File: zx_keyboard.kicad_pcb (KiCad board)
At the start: 2 copper layers, 194.3 x 127 mm, 3 parts, among them SW1 SW_PUSH, SW2 SW_PUSH, U1 4066

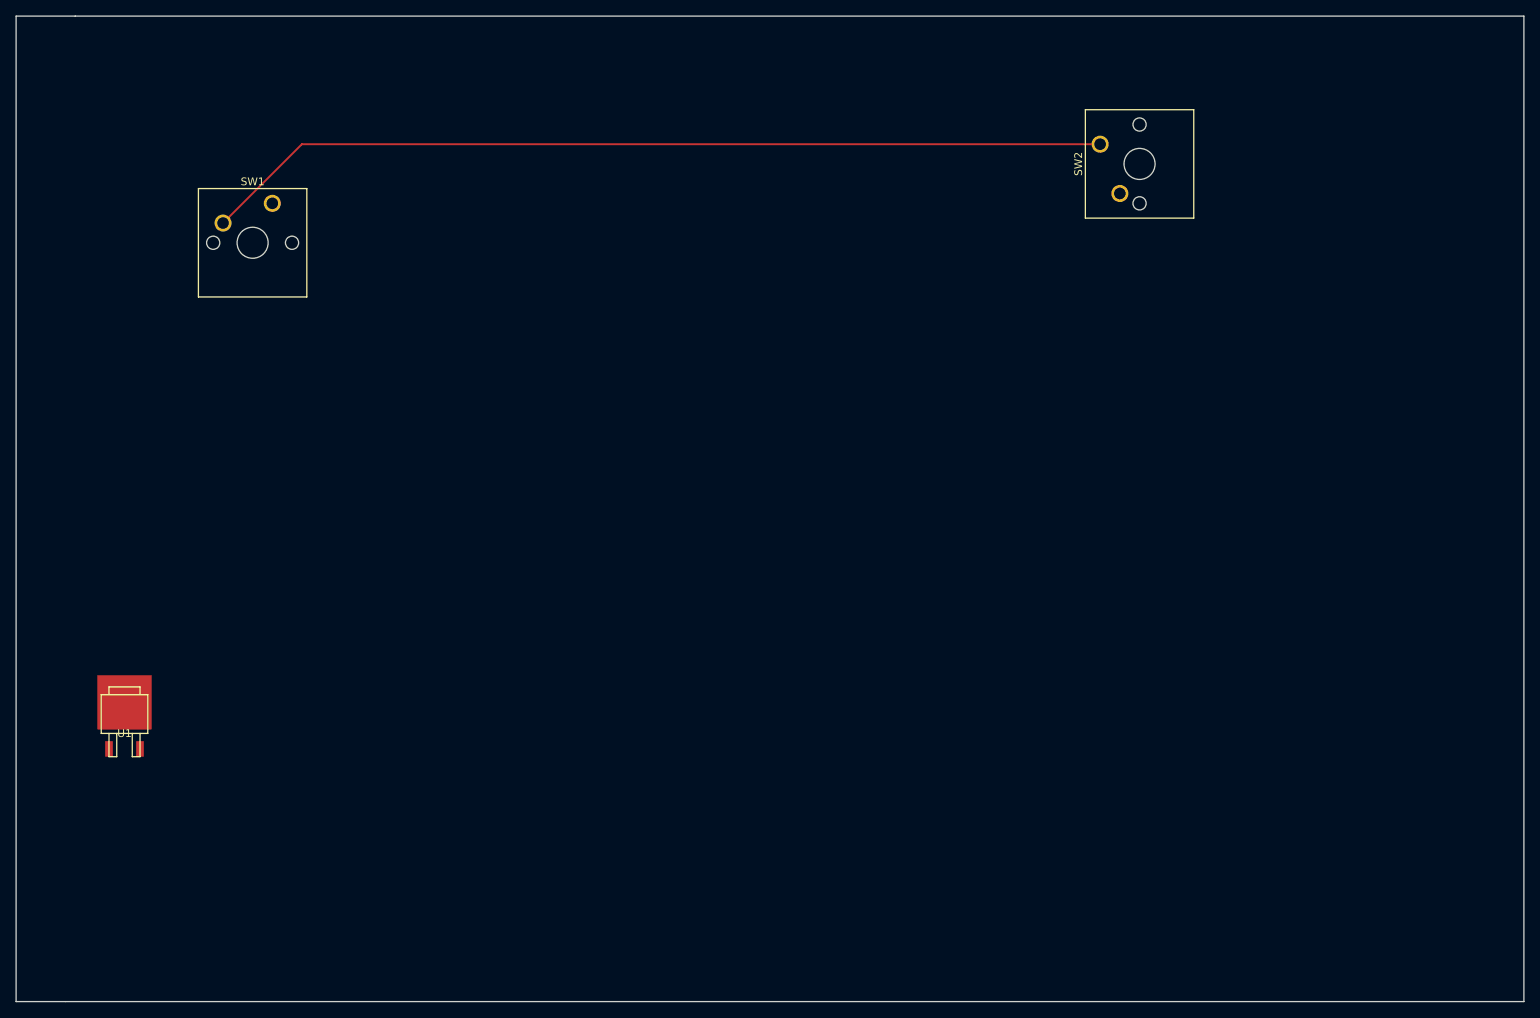
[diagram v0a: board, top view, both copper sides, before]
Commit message: pcb
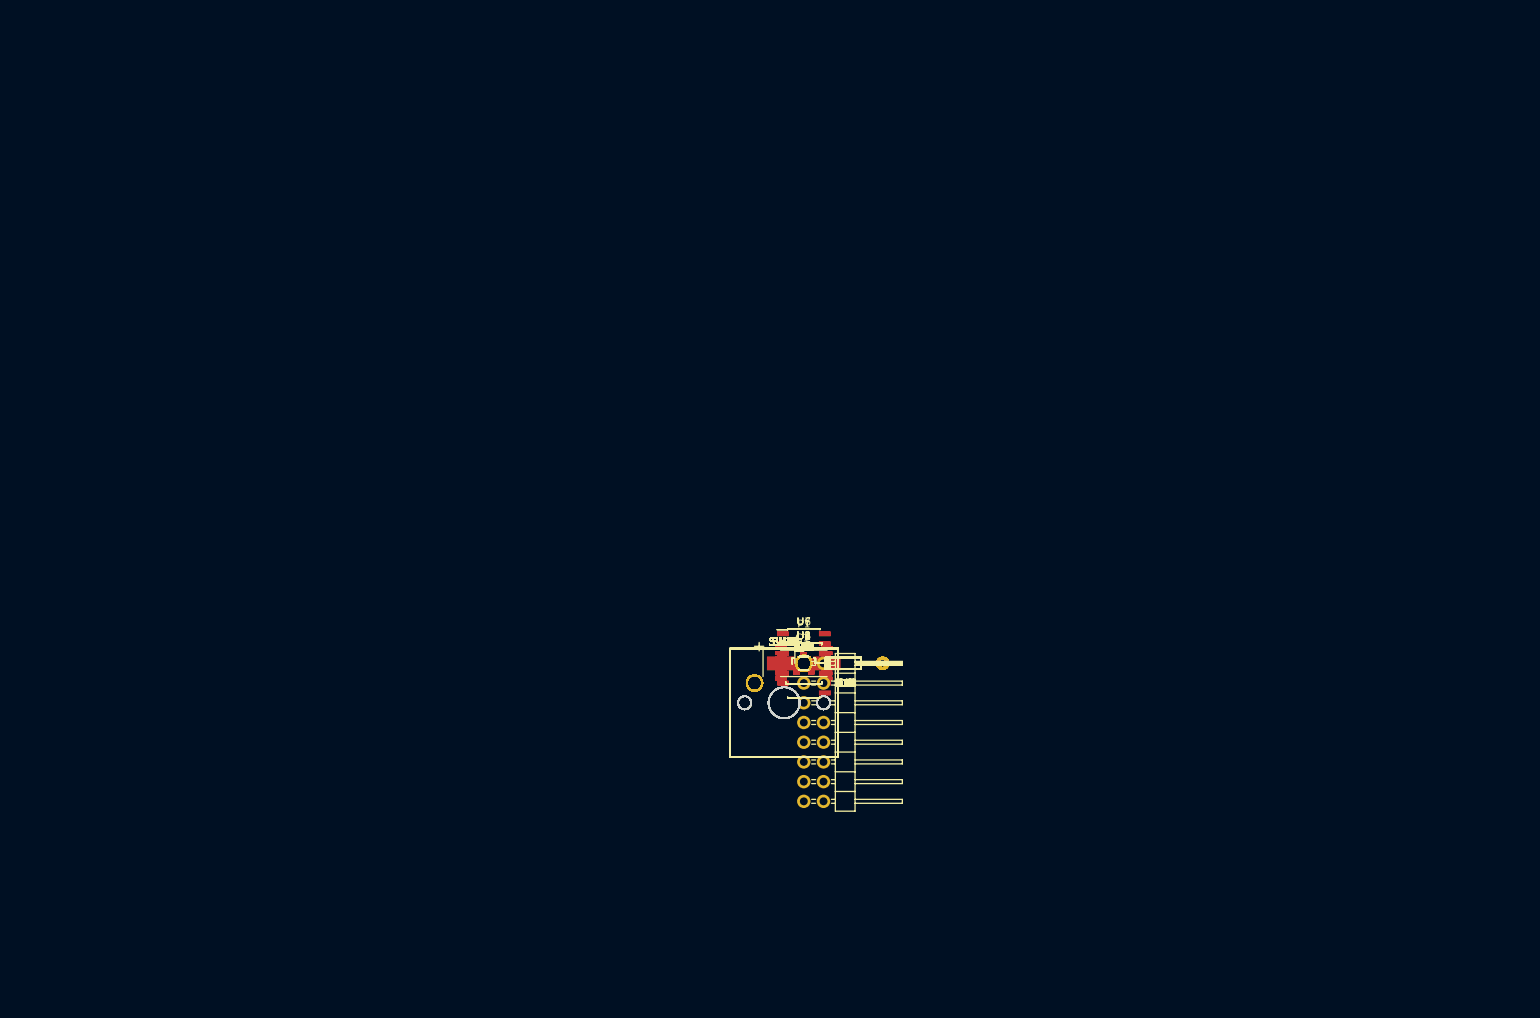
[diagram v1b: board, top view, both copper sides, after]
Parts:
- added C1: 10uF, Capacitors_Tantalum_SMD:TantalC_SizeC_EIA-6032_HandSoldering, F.Cu at (148.5, 105.0)
- added D1, D10, D11, D12, D13, D14, D15, D16, D17, D2, D3, D4, D5, D6, D7, D8, D9: BAT41, Diodes_ThroughHole:Diode_DO-35_SOD27_Horizontal_RM10, F.Cu at (148.5, 105.0)
- added P1: CONN_02X08, Pin_Headers:Pin_Header_Angled_2x08, F.Cu at (148.5, 105.0)
- added Q1, Q2, Q3, Q4, Q5, Q6, Q7, Q8: BSS123, TO_SOT_Packages_SMD:SOT-23, F.Cu at (148.5, 105.0)
- added R1, R11, R13, R15, R17, R19, R2, R21, R23, R25, R27, R29, R3, R31, R33, R35, R37, R39, R4, R5, R7, R9: 10K, Resistors_SMD:R_0805_HandSoldering, F.Cu at (148.5, 105.0)
- added R10, R12, R14, R16, R18, R20, R22, R24, R26, R28, R30, R32, R34, R36, R38, R40, R41, R42, R43, R44, R6, R8: 1K, Resistors_SMD:R_0805_HandSoldering, F.Cu at (148.5, 105.0)
- added R45, R46, R47, R48, R49, R50, R51, R52: 100, Resistors_SMD:R_0805_HandSoldering, F.Cu at (148.5, 105.0)
- added SW10: KEY_0, Buttons_Switches_Keyboard:SW_Cherry_MX1A_1.00u_PCB, F.Cu at (148.5, 105.0)
- added SW11: KEY_Q, Buttons_Switches_Keyboard:SW_Cherry_MX1A_1.00u_PCB, F.Cu at (148.5, 105.0)
- added SW12: KEY_W, Buttons_Switches_Keyboard:SW_Cherry_MX1A_1.00u_PCB, F.Cu at (148.5, 105.0)
- added SW13: KEY_E, Buttons_Switches_Keyboard:SW_Cherry_MX1A_1.00u_PCB, F.Cu at (148.5, 105.0)
- added SW14: KEY_R, Buttons_Switches_Keyboard:SW_Cherry_MX1A_1.00u_PCB, F.Cu at (148.5, 105.0)
- added SW15: KEY_T, Buttons_Switches_Keyboard:SW_Cherry_MX1A_1.00u_PCB, F.Cu at (148.5, 105.0)
- added SW16: KEY_Y, Buttons_Switches_Keyboard:SW_Cherry_MX1A_1.00u_PCB, F.Cu at (148.5, 105.0)
- added SW17: KEY_U, Buttons_Switches_Keyboard:SW_Cherry_MX1A_1.00u_PCB, F.Cu at (148.5, 105.0)
- added SW18: KEY_I, Buttons_Switches_Keyboard:SW_Cherry_MX1A_1.00u_PCB, F.Cu at (148.5, 105.0)
- added SW19: KEY_O, Buttons_Switches_Keyboard:SW_Cherry_MX1A_1.00u_PCB, F.Cu at (148.5, 105.0)
- added SW20: KEY_P, Buttons_Switches_Keyboard:SW_Cherry_MX1A_1.00u_PCB, F.Cu at (148.5, 105.0)
- added SW21: KEY_A, Buttons_Switches_Keyboard:SW_Cherry_MX1A_1.00u_PCB, F.Cu at (148.5, 105.0)
- added SW22: KEY_S, Buttons_Switches_Keyboard:SW_Cherry_MX1A_1.00u_PCB, F.Cu at (148.5, 105.0)
- added SW23: KEY_D, Buttons_Switches_Keyboard:SW_Cherry_MX1A_1.00u_PCB, F.Cu at (148.5, 105.0)
- added SW24: KEY_F, Buttons_Switches_Keyboard:SW_Cherry_MX1A_1.00u_PCB, F.Cu at (148.5, 105.0)
- added SW25: KEY_G, Buttons_Switches_Keyboard:SW_Cherry_MX1A_1.00u_PCB, F.Cu at (148.5, 105.0)
- added SW26: KEY_H, Buttons_Switches_Keyboard:SW_Cherry_MX1A_1.00u_PCB, F.Cu at (148.5, 105.0)
- added SW27: KEY_J, Buttons_Switches_Keyboard:SW_Cherry_MX1A_1.00u_PCB, F.Cu at (148.5, 105.0)
- added SW28: KEY_K, Buttons_Switches_Keyboard:SW_Cherry_MX1A_1.00u_PCB, F.Cu at (148.5, 105.0)
- added SW29: KEY_L, Buttons_Switches_Keyboard:SW_Cherry_MX1A_1.00u_PCB, F.Cu at (148.5, 105.0)
- added SW3: KEY_3, Buttons_Switches_Keyboard:SW_Cherry_MX1A_1.00u_PCB, F.Cu at (148.5, 105.0)
- added SW30: KEY_EN, Buttons_Switches_Keyboard:SW_Cherry_MX1A_1.00u_PCB, F.Cu at (148.5, 105.0)
- added SW31: KEY_CS1, Buttons_Switches_Keyboard:SW_Cherry_MX1A_1.00u_PCB, F.Cu at (148.5, 105.0)
- added SW32: KEY_Z, Buttons_Switches_Keyboard:SW_Cherry_MX1A_1.00u_PCB, F.Cu at (148.5, 105.0)
- added SW33: KEY_X, Buttons_Switches_Keyboard:SW_Cherry_MX1A_1.00u_PCB, F.Cu at (148.5, 105.0)
- added SW34: KEY_C, Buttons_Switches_Keyboard:SW_Cherry_MX1A_1.00u_PCB, F.Cu at (148.5, 105.0)
- added SW35: KEY_V, Buttons_Switches_Keyboard:SW_Cherry_MX1A_1.00u_PCB, F.Cu at (148.5, 105.0)
- added SW36: KEY_B, Buttons_Switches_Keyboard:SW_Cherry_MX1A_1.00u_PCB, F.Cu at (148.5, 105.0)
- added SW37: KEY_N, Buttons_Switches_Keyboard:SW_Cherry_MX1A_1.00u_PCB, F.Cu at (148.5, 105.0)
- added SW38: KEY_M, Buttons_Switches_Keyboard:SW_Cherry_MX1A_1.00u_PCB, F.Cu at (148.5, 105.0)
- added SW39: KEY_SS1, Buttons_Switches_Keyboard:SW_Cherry_MX1A_1.00u_PCB, F.Cu at (148.5, 105.0)
- added SW4: KEY_4, Buttons_Switches_Keyboard:SW_Cherry_MX1A_1.00u_PCB, F.Cu at (148.5, 105.0)
- added SW40: KEY_SP, Buttons_Switches_Keyboard:SW_Cherry_MX1A_1.00u_PCB, F.Cu at (148.5, 105.0)
- added SW41: KEY_CS2, Buttons_Switches_Keyboard:SW_Cherry_MX1A_1.00u_PCB, F.Cu at (148.5, 105.0)
- added SW42: KEY_SS2, Buttons_Switches_Keyboard:SW_Cherry_MX1A_1.00u_PCB, F.Cu at (148.5, 105.0)
- added SW43: KEY_EDIT, Buttons_Switches_Keyboard:SW_Cherry_MX1A_1.00u_PCB, F.Cu at (148.5, 105.0)
- added SW44: KEY_CL, Buttons_Switches_Keyboard:SW_Cherry_MX1A_1.00u_PCB, F.Cu at (148.5, 105.0)
- added SW45: KEY_TV, Buttons_Switches_Keyboard:SW_Cherry_MX1A_1.00u_PCB, F.Cu at (148.5, 105.0)
- added SW46: KEY_IV, Buttons_Switches_Keyboard:SW_Cherry_MX1A_1.00u_PCB, F.Cu at (148.5, 105.0)
- added SW47: KEY_LEFT, Buttons_Switches_Keyboard:SW_Cherry_MX1A_1.00u_PCB, F.Cu at (148.5, 105.0)
- added SW48: KEY_DOWN, Buttons_Switches_Keyboard:SW_Cherry_MX1A_1.00u_PCB, F.Cu at (148.5, 105.0)
- added SW49: KEY_UP, Buttons_Switches_Keyboard:SW_Cherry_MX1A_1.00u_PCB, F.Cu at (148.5, 105.0)
- added SW5: KEY_5, Buttons_Switches_Keyboard:SW_Cherry_MX1A_1.00u_PCB, F.Cu at (148.5, 105.0)
- added SW50: KEY_RIGHT, Buttons_Switches_Keyboard:SW_Cherry_MX1A_1.00u_PCB, F.Cu at (148.5, 105.0)
- added SW51: KEY_GR, Buttons_Switches_Keyboard:SW_Cherry_MX1A_1.00u_PCB, F.Cu at (148.5, 105.0)
- added SW52: KEY_DEL, Buttons_Switches_Keyboard:SW_Cherry_MX1A_1.00u_PCB, F.Cu at (148.5, 105.0)
- added SW53: KEY_QUOT, Buttons_Switches_Keyboard:SW_Cherry_MX1A_1.00u_PCB, F.Cu at (148.5, 105.0)
- added SW54: KEY_SEM, Buttons_Switches_Keyboard:SW_Cherry_MX1A_1.00u_PCB, F.Cu at (148.5, 105.0)
- added SW55: KEY_BREAK, Buttons_Switches_Keyboard:SW_Cherry_MX1A_1.00u_PCB, F.Cu at (148.5, 105.0)
- added SW56: KEY_DOT, Buttons_Switches_Keyboard:SW_Cherry_MX1A_1.00u_PCB, F.Cu at (148.5, 105.0)
- added SW57: KEY_COMMA, Buttons_Switches_Keyboard:SW_Cherry_MX1A_1.00u_PCB, F.Cu at (148.5, 105.0)
- added SW58: KEY_EXT, Buttons_Switches_Keyboard:SW_Cherry_MX1A_1.00u_PCB, F.Cu at (148.5, 105.0)
- added SW6: KEY_6, Buttons_Switches_Keyboard:SW_Cherry_MX1A_1.00u_PCB, F.Cu at (148.5, 105.0)
- added SW7: KEY_7, Buttons_Switches_Keyboard:SW_Cherry_MX1A_1.00u_PCB, F.Cu at (148.5, 105.0)
- added SW8: KEY_8, Buttons_Switches_Keyboard:SW_Cherry_MX1A_1.00u_PCB, F.Cu at (148.5, 105.0)
- added SW9: KEY_9, Buttons_Switches_Keyboard:SW_Cherry_MX1A_1.00u_PCB, F.Cu at (148.5, 105.0)
- added U2, U3, U4, U5: 4066, Housings_SSOP:TSSOP-14_4.4x5mm_Pitch0.65mm, F.Cu at (148.5, 105.0)
- added U6, U7: 74HC14, Housings_SOIC:SOIC-14_3.9x8.7mm_Pitch1.27mm, F.Cu at (148.5, 105.0)
- SW1: value SW_PUSH -> KEY_1
- SW2: value SW_PUSH -> KEY_2
- U1: footprint TO_SOT_Packages_SMD:SOT-428 -> Housings_SSOP:TSSOP-14_4.4x5mm_Pitch0.65mm
- moved SW1 90.6 mm to (148.5, 105.0)
- moved U1 87.9 mm to (148.5, 105.0)
- moved SW2 77.0 mm to (148.5, 105.0), turned to 0 degrees
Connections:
- SW1 pad 1: Net-(SW1-Pad1) -> /KA11
- SW1 pad 2: Net-(SW1-Pad2) -> /KD0
- SW2 pad 1: Net-(SW1-Pad2) -> /KA11
- SW2 pad 2: Net-(SW2-Pad2) -> /KD1
- U1 pad 1: Net-(U1-Pad1) -> /KD0
- U1 pad 2: Net-(U1-Pad13) -> /KA11
- U1 pad 3: Net-(U1-Pad14) -> /KA11
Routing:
- net Net-(SW1-Pad2): track 117.2 -> 0.00 mm
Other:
- board outline removed
- rule pad_to_mask_clearance: 0.2 -> 0
